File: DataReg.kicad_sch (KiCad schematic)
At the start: 39 parts, among them U10 74LVC574AD, U11 74LVC574AD, U12 74LVC574AD, U13 74LVC574AD, U29 74LVC574AD, U30 74LVC574AD, U31 74LVC574AD, U32 74LVC574AD, U33 74LVC574AD, U35 74LVC74AD, U38 74LVC574AD, U39 74LVC574AD, U40 74LVC574AD, U41 74LVC574AD, U42 74LVC32AD, U5 74LVC574AD, U6 74LVC574AD, U7 74LVC574AD, U8 74LVC574AD, U9 74LVC574AD

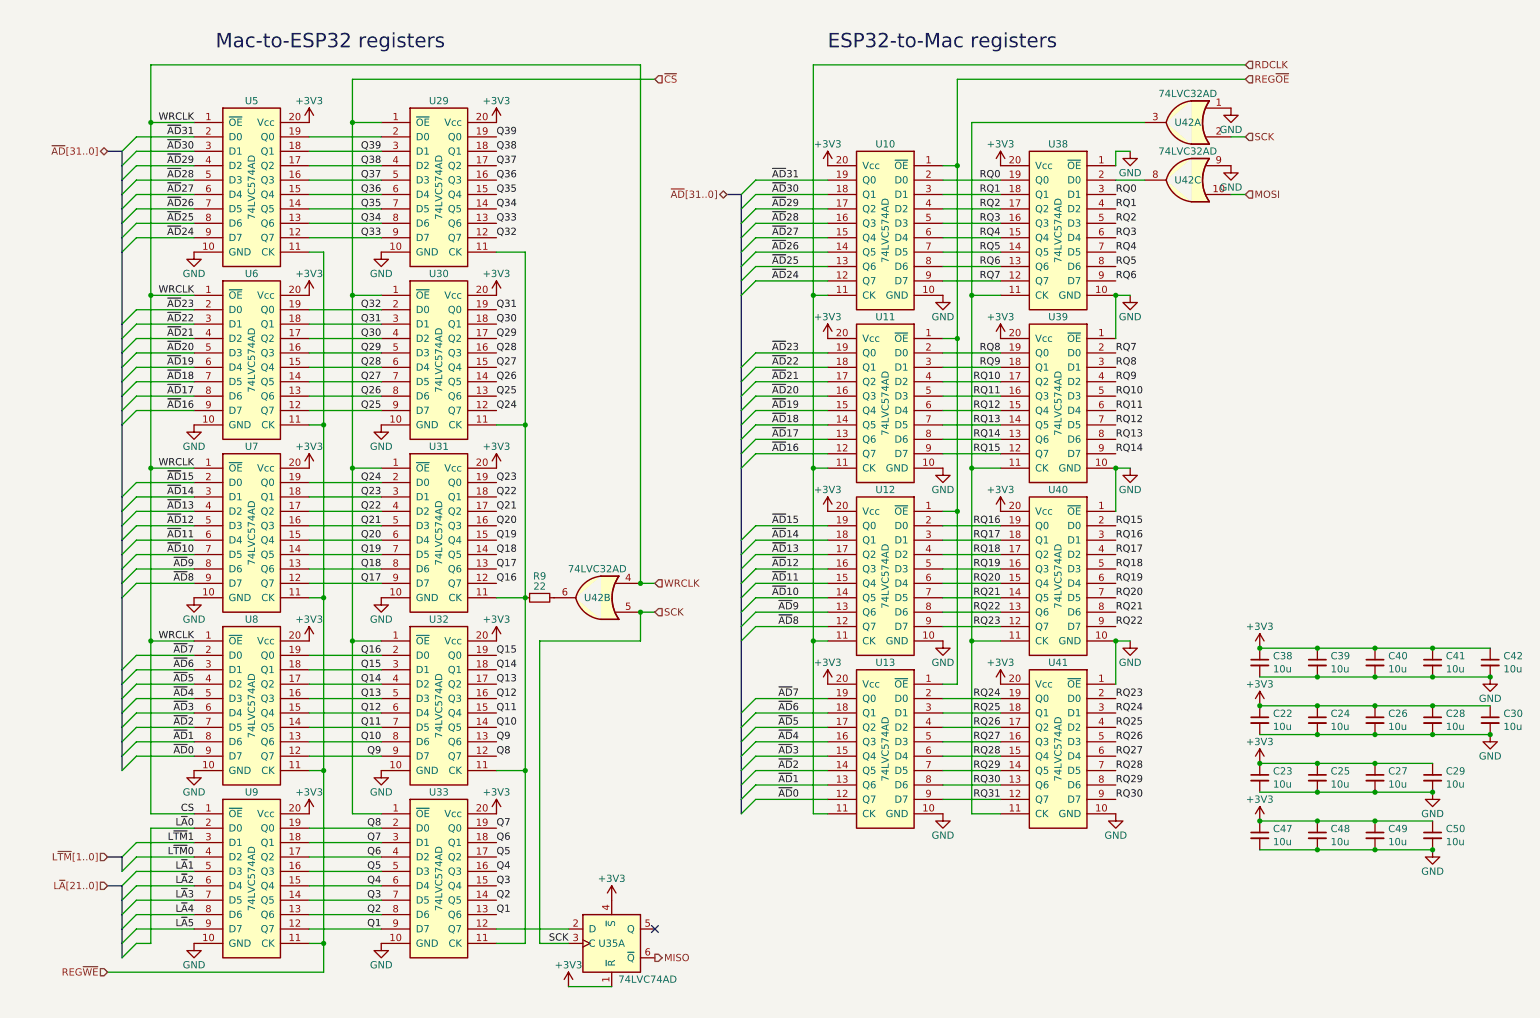
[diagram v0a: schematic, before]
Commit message: did I mess this up?
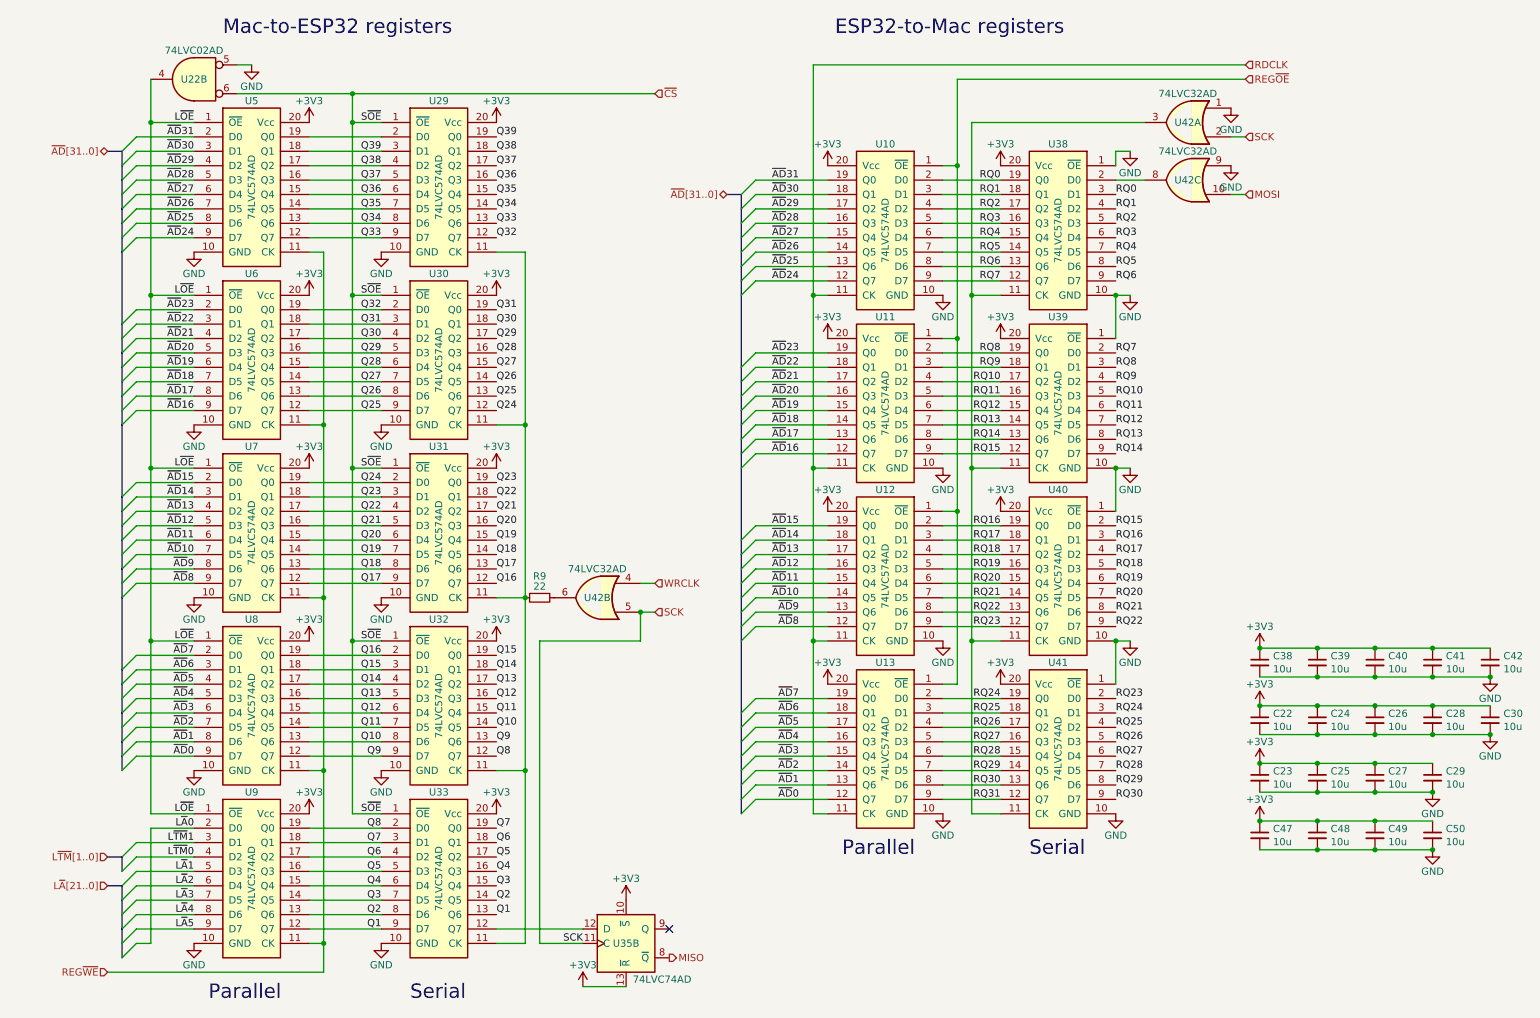
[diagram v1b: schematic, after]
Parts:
- added U22: 74LVC02AD, stdpads:SOIC-14_3.9mm, symbol 74xx:74LS02
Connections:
- net +3V3: now also U35.10 (~{S}), U35.13 (~{R}); no longer U35.1 (~{R}), U35.4 (~{S})
- net GND: now also U22.5
- net MISO: now also U35.8 (~{Q}); no longer U35.6 (~{Q})
- net SCK: now also U35.11 (C); no longer U35.3 (C)
- net WRCLK: no longer U5.1 (~{OE}), U6.1 (~{OE}), U7.1 (~{OE}), U8.1 (~{OE}), U9.1 (~{OE})
- net ~{CS}: now also U22.6
- net at U33.12 (Q7): now also U35.12 (D); no longer U35.2 (D)
- new net L~{OE}: U22.4, U5.1 (~{OE}), U6.1 (~{OE}), U7.1 (~{OE}), U8.1 (~{OE}), U9.1 (~{OE})
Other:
- note added: "Parallel"
- note added: "Serial"
- moved on the sheet: U35B

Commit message: Revert "did I mess this up?"
This reverts commit fd75c937204418059e97b488ea791750328fc4dd.
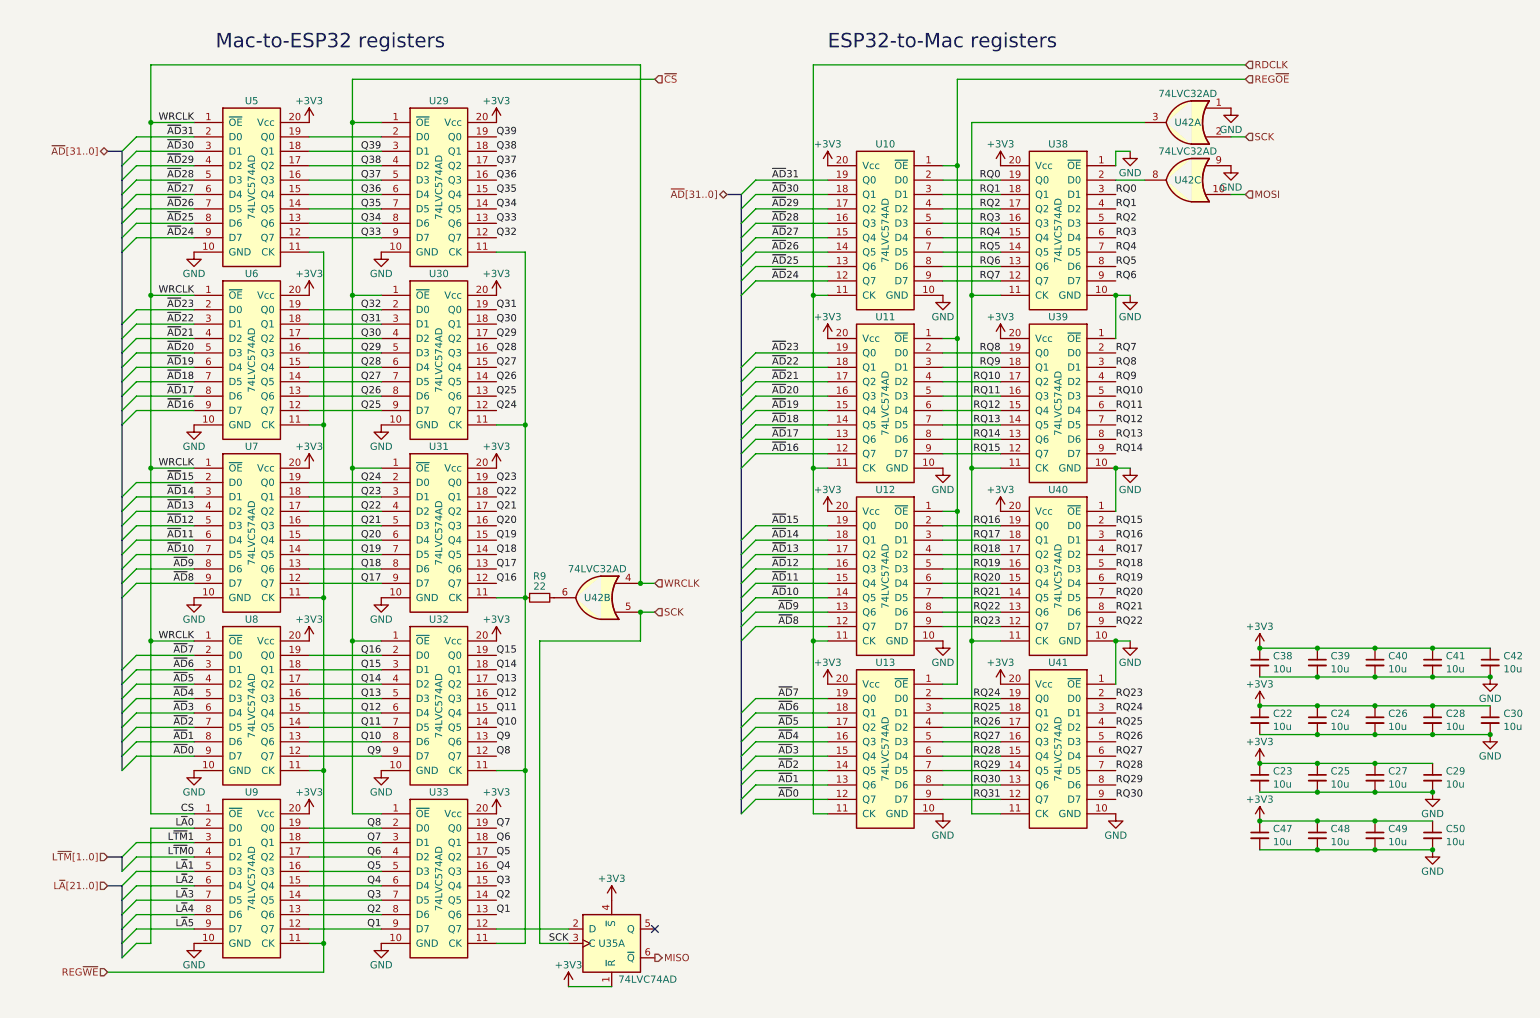
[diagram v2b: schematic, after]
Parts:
- removed U22: 74LVC02AD, stdpads:SOIC-14_3.9mm, symbol 74xx:74LS02
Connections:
- net L~{OE} is gone; now on net WRCLK: U5.1 (~{OE}), U6.1 (~{OE}), U7.1 (~{OE}), U8.1 (~{OE}), U9.1 (~{OE})
- net +3V3: now also U35.1 (~{R}), U35.4 (~{S}); no longer U35.10 (~{S}), U35.13 (~{R})
- net MISO: now also U35.6 (~{Q}); no longer U35.8 (~{Q})
- net SCK: now also U35.3 (C); no longer U35.11 (C)
- net at U33.12 (Q7): now also U35.2 (D); no longer U35.12 (D)
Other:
- note removed: "Parallel"
- note removed: "Serial"
- moved on the sheet: U35A
